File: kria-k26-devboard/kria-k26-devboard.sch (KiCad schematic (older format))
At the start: 0 parts

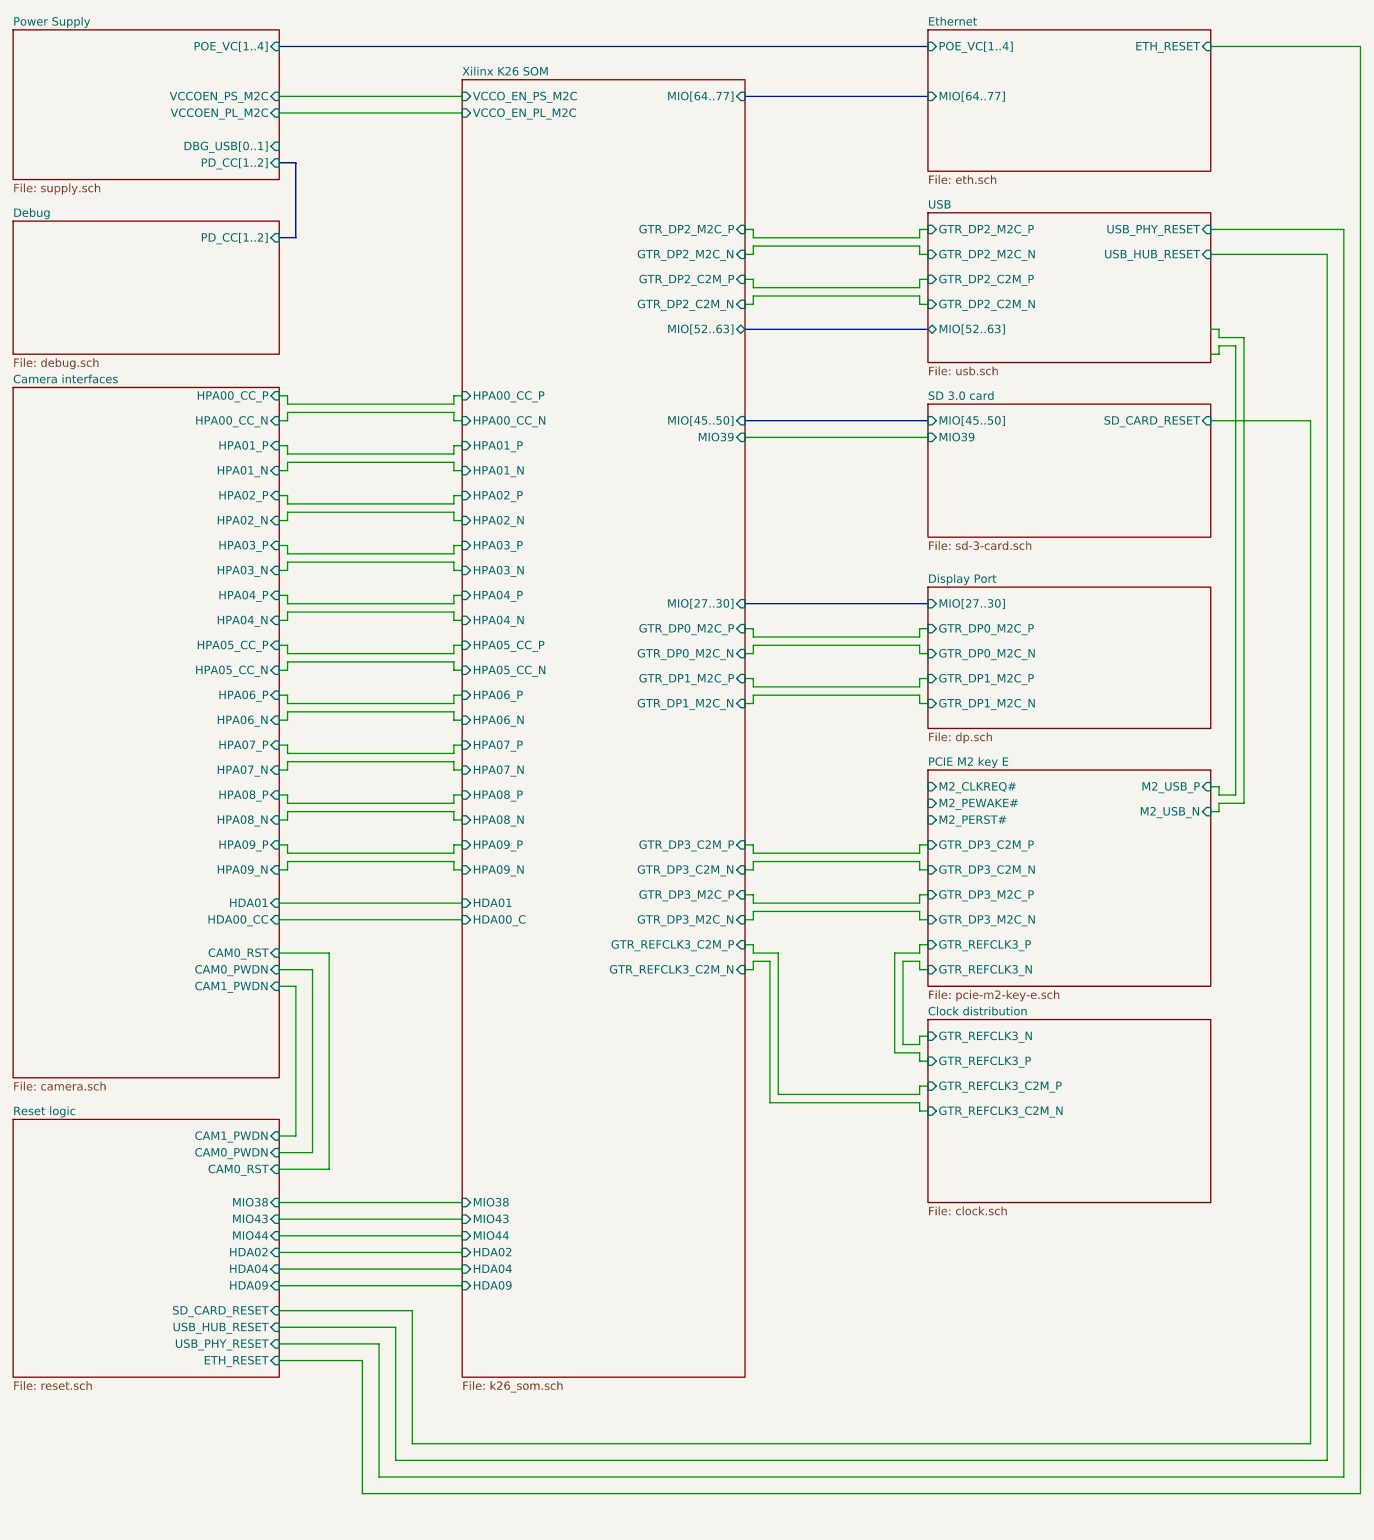
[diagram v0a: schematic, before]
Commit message: Progress on Debug sheet
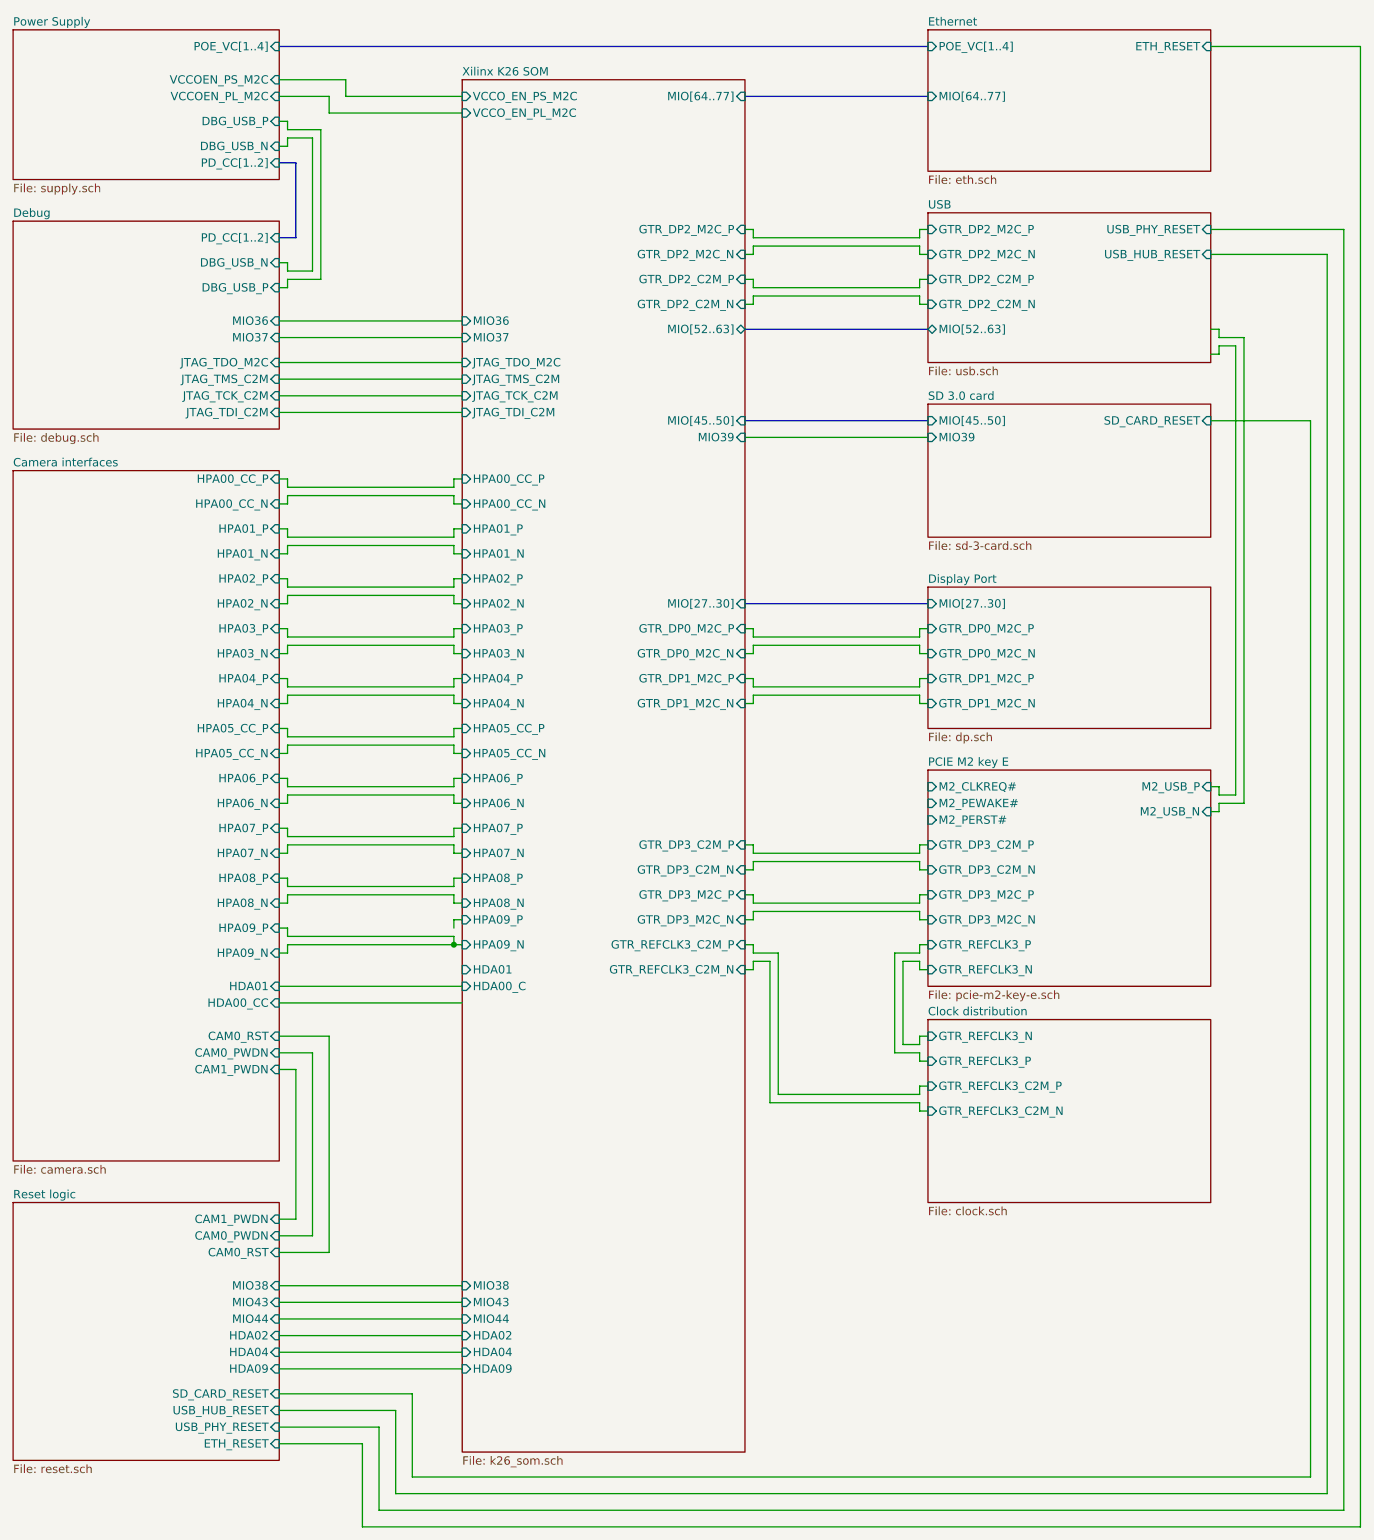
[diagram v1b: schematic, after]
